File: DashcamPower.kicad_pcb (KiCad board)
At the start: 6 copper layers, 48 x 17.5 mm, 53 parts, among them J1 USB_C_Receptacle_USB2.0_16P, J2 USB_C_Receptacle_USB2.0_16P, J4 Conn_01x06, Q1 IRLML6402, Q2 MMBT5551L, Q3 MMBT5551L, SW1 B3FS-1000P, U1 XC6206P332MR-G, U2 LSM6DS3, U3 RP2040, U4 W25Q128JVS, Y1 X322512MSB4SI

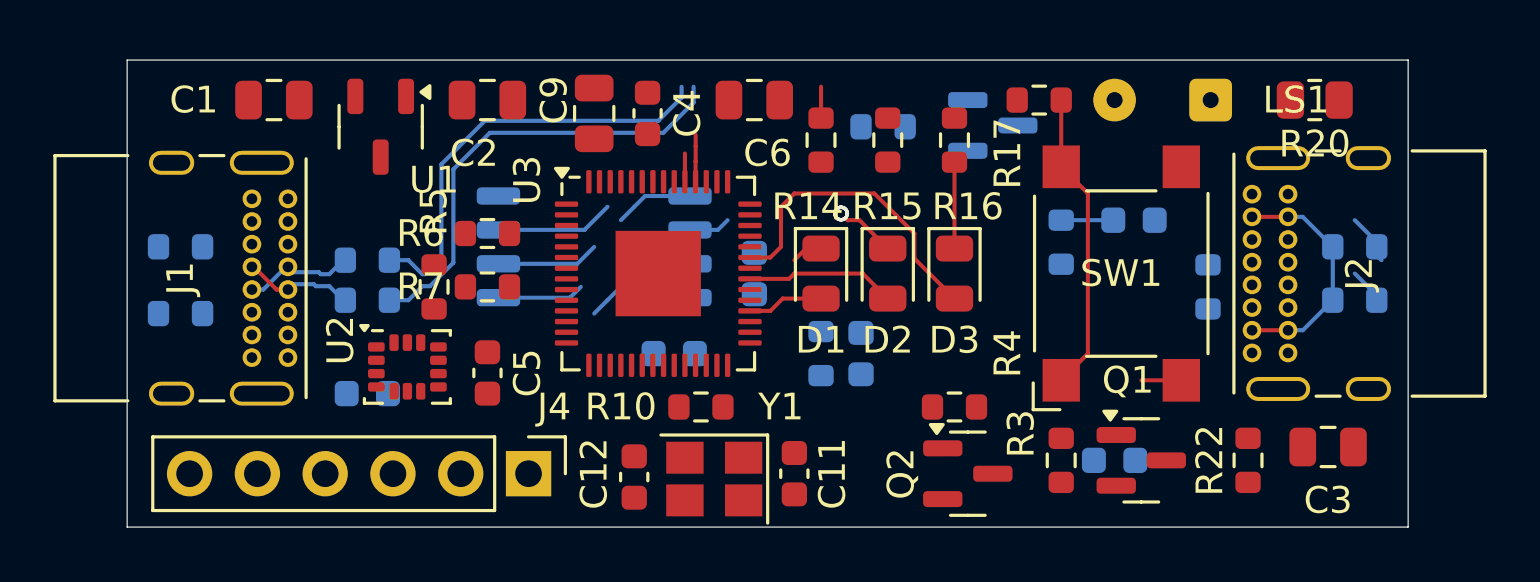
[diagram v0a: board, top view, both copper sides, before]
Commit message: Ready to alter IMU
Ready to alter IMU
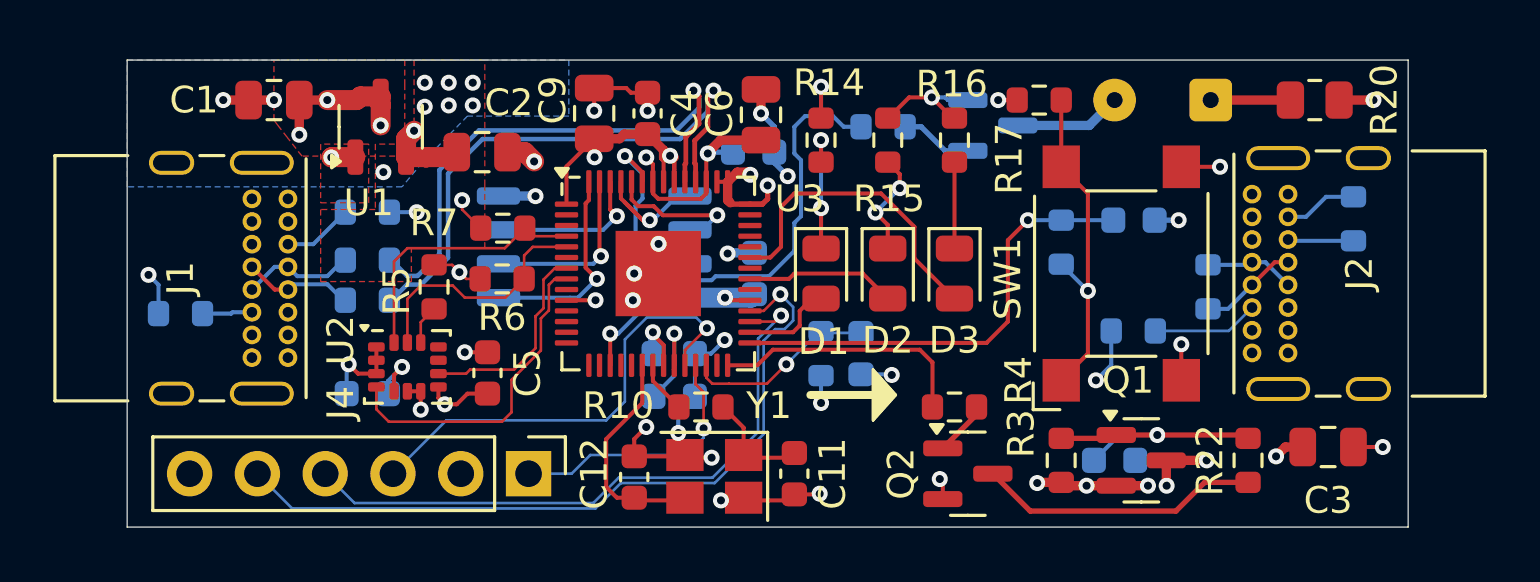
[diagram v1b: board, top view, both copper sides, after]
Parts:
- added C16: 100n, Capacitor_SMD:C_0603_1608Metric, B.Cu at (88.0, 104.6)
- added C17: 100n, Capacitor_SMD:C_0603_1608Metric, B.Cu at (91.0, 95.5)
- moved R12 8.88 mm to (105.2, 102.2)
- moved R2 7.12 mm to (76.5, 97.7), turned to 0 degrees
- moved R11 3.05 mm to (113.5, 98.0), turned to -90 degrees
- moved R7 2.27 mm to (81.6, 98.3)
- moved C2 1.96 mm to (80.8, 95.5), turned to 0 degrees
- moved R6 1.79 mm to (81.5, 100.2)
- moved C6 0.60 mm to (91.2, 94.0), turned to 90 degrees
- moved Y1 0.10 mm to (89.5, 107.6)
- turned U1 to 90 degrees
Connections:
- net Net-(Q1-D) renamed /USB_VOUT
- net Net-(U3-VREG_VOUT) renamed /VCORE
- U3 pad 11: /BTN -> unconnected-(U3-GPIO8-Pad11)
- U3 pad 2: /USB_OUT_ON -> unconnected-(U3-GPIO0-Pad2)
- U3 pad 28: unconnected-(U3-GPIO17-Pad28) -> /USB_OUT_ON
- U3 pad 29: unconnected-(U3-GPIO18-Pad29) -> /BTN
- U3 pad 30: unconnected-(U3-GPIO19-Pad30) -> /LED_G
- U3 pad 31: unconnected-(U3-GPIO20-Pad31) -> /UTX
- U3 pad 32: /LED_G -> /URX
- U3 pad 7: /IMU_INT1 -> /IMU_INT2
- U3 pad 8: /IMU_INT2 -> /IMU_INT1
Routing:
- net GND: track 2.67 -> 51.2 mm, vias 0 -> 32
- net +3.3V: track 0.00 -> 33.5 mm, vias 0 -> 21
- net /URX: track 0.00 -> 28.3 mm, vias 0 -> 1
- net /UTX: track 0.00 -> 23.8 mm, vias 0 -> 1
- net /SWC: track 0.00 -> 17.4 mm, vias 0 -> 1
- net /BUZZER: track 0.00 -> 17.1 mm, vias 0 -> 1
- net /BTN: track 1.95 -> 17.3 mm, vias 0 -> 1
- net /VCORE: track 0.00 -> 12.4 mm, vias 0 -> 3
- net /IMU_INT1: track 0.00 -> 12.3 mm
- net +5V: track 0.00 -> 11.1 mm, vias 0 -> 7
- net Net-(Q2-C): track 0.00 -> 10.6 mm
- net /I2C_SDA: track 0.00 -> 10.1 mm
- net /SWD: track 0.00 -> 9.96 mm, vias 0 -> 1
- net Net-(Q1-G): track 0.00 -> 9.87 mm, vias 0 -> 1
- net /USB_OUT_ON: track 0.00 -> 9.79 mm
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- added copper zone on B.Cu, net +3.3V
- added copper zone on F.Cu, net +3.3V
- added copper zone on In3.Cu, net +3.3V
- added copper zone on F.Cu, net +5V
- added copper zone on In2.Cu, net +5V
- added copper zone on In1.Cu, net /USB_VOUT
- added copper zone on In2.Cu, net /VCORE
- added copper zone on F.Cu, net GND
- added copper zone on In1.Cu, net GND
- added copper zone on In4.Cu, net GND
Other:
- board text added: "DashcamPwr"
- board text added: "TGO 2025"
